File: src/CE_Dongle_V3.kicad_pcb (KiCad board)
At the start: 4 copper layers, 44 x 44 mm, 110 parts, among them J1 USB_C_Receptacle_USB2.0_16P, J2 8P8C_LED_Shielded, J3 Conn_Coaxial, J4 Conn_02x05_Odd_Even, J5 Conn_01x02, Q1 AO3401A, Q2 AO3401A, Q3 BC817-40-7-F, Q4 BC817-40-7-F, Q5 BC817-40-7-F, U1 ESP32-C6, U10 TMUX1208QRSVRQ1, U11 TPS70950DBVR, U2 SP3485, U3 W25Q64JWUUIQ, U4 TPS54302DDCR, U5 PCF8574RGTR(UMW), U6 PCF8574RGTR(UMW), U7 TMUX1208QRSVRQ1, U8 TMUX1208QRSVRQ1, U9 TMUX1208QRSVRQ1, Y1 40MHz

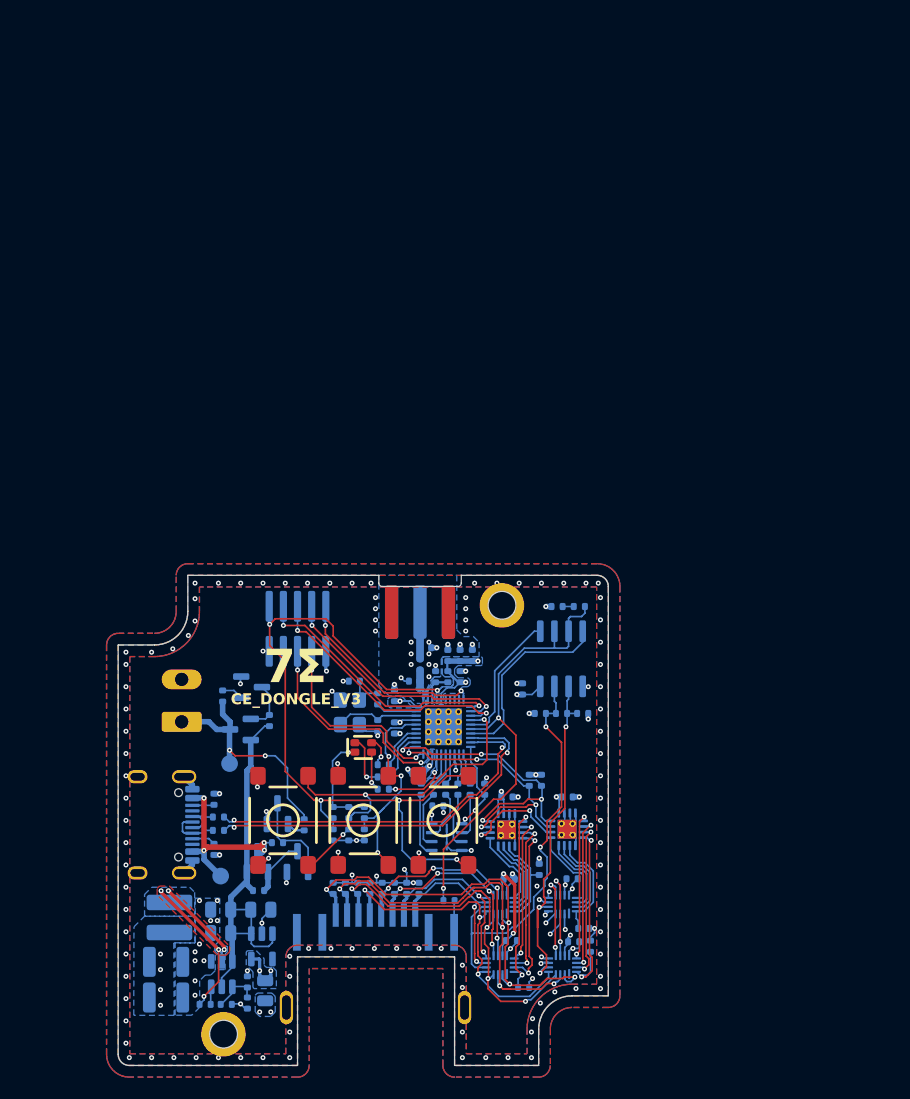
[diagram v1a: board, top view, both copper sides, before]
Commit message: ongoing work
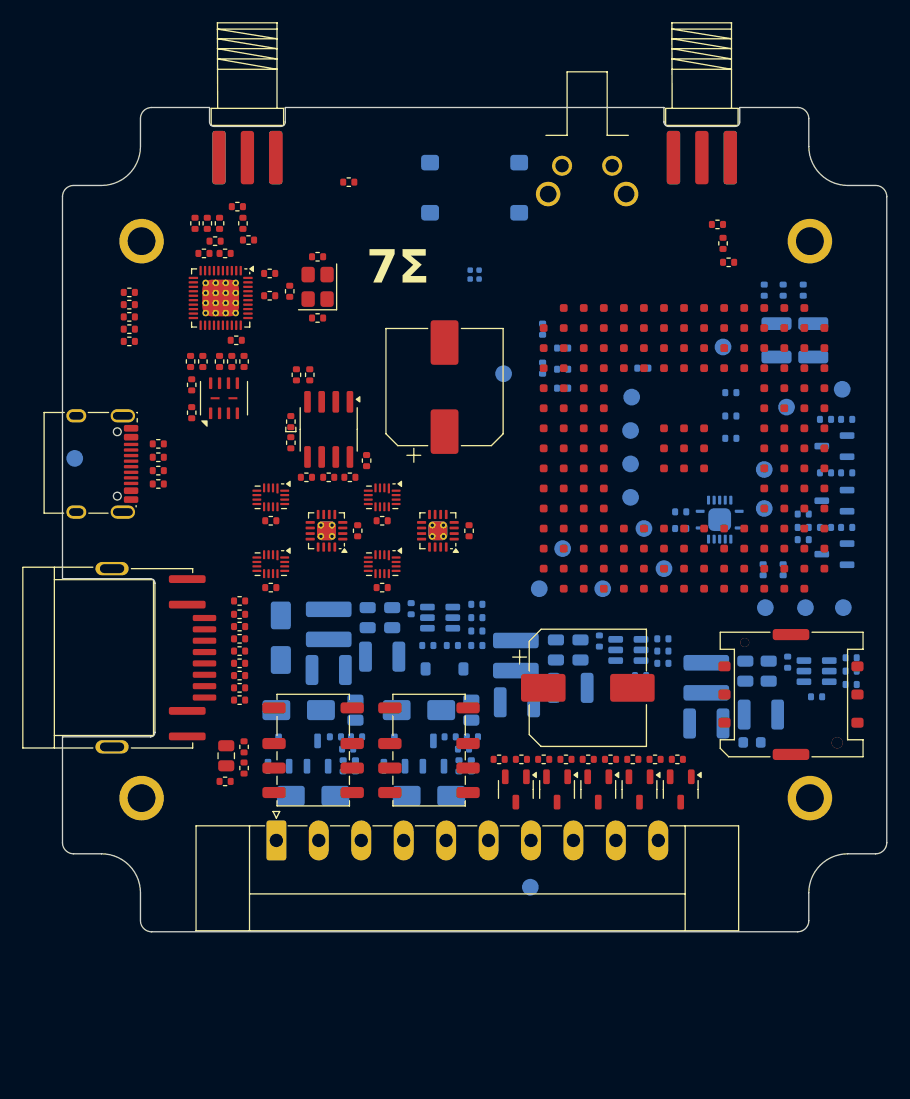
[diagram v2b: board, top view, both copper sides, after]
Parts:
- removed D7: XL-3227SURUGC, 7Sigma:LED-SMD_4P-L1.6-W1.5-BR
- removed G2: Hammond_1551RFLGY, 7Sigma:HAMMOND_1551RFLGY
- removed J2: 8P8C_LED_Shielded, 7Sigma:RJ45-TH_RC01812
- removed J3: Conn_Coaxial, 7Sigma:SMA-SMD_BWSMA-KE-P001
- removed Q3, Q4, Q5: BC817-40-7-F, 7Sigma:SOT-23
- removed R19, R23, R24: 120R, 7Sigma:R_0402_1005Metric
- removed R41: 100K, 7Sigma:R_0402_1005Metric
- removed SW_BOOT1, SW_RST1, SW_USR1: KH-6X6X4.3H-STM, 7Sigma:SW-SMD_4P-L6.0-W6.0-P4.50-LS9.0-H4.3
- removed U11: TPS70950DBVR, 7Sigma:SOT-23-5
- added C40: 100nF, 7Sigma:C_0402_1005Metric, B.Cu at (170.7, 115.9)
- added C41: 220pF, 7Sigma:C_0402_1005Metric, B.Cu at (173.8, 113.6)
- added C42: 47uF, 7Sigma:C_1210_3225Metric, B.Cu at (160.8, 118.3)
- added C43: 47uF, 7Sigma:C_1210_3225Metric, B.Cu at (165.7, 117.5)
- added C44: 470uF, 7Sigma:CP_Elec_10x10, F.Cu at (150.2, 115.1)
- added C45: 470uF, 7Sigma:CP_Elec_10x10, F.Cu at (137.3, 88.1)
- added C48: 100nF, 7Sigma:C_0402_1005Metric, B.Cu at (166.0, 79.4)
- added C49: 100nF, 7Sigma:C_0402_1005Metric, B.Cu at (167.7, 79.4)
- added C50: 100nF, 7Sigma:C_0402_1005Metric, B.Cu at (158.5, 99.3)
- added C51: 100nF, 7Sigma:C_0402_1005Metric, B.Cu at (158.5, 100.8)
- added C52: 10nF, 7Sigma:C_0402_1005Metric, B.Cu at (169.5, 101.8)
- added C53: 10nF, 7Sigma:C_0402_1005Metric, B.Cu at (169.5, 99.5)
- added C54: 100nF, 7Sigma:C_0402_1005Metric, B.Cu at (169.5, 79.4)
- added C62: 33pF, 7Sigma:C_0402_1005Metric, B.Cu at (167.7, 104.5)
- added C63: 33pF, 7Sigma:C_0402_1005Metric, B.Cu at (165.9, 104.5)
- added C64: 1uF, 7Sigma:C_0402_1005Metric, B.Cu at (146.1, 82.9)
- added C65: 33pF, 7Sigma:C_0402_1005Metric, B.Cu at (147.9, 88.2)
- added C66: 100nF, 7Sigma:C_0402_1005Metric, B.Cu at (147.9, 84.6)
- added C67: 33pF, 7Sigma:C_0402_1005Metric, B.Cu at (163.0, 88.6)
- added C68: 33pF, 7Sigma:C_0402_1005Metric, B.Cu at (163.0, 90.7)
- added C69: 33pF, 7Sigma:C_0402_1005Metric, B.Cu at (163.0, 92.7)
- added C70: 1.2pF, 7Sigma:C_0402_1005Metric, F.Cu at (162.8, 76.9)
- added C71: 1.2pF, 7Sigma:C_0402_1005Metric, F.Cu at (161.8, 73.5)
- added C78: 47uF, 7Sigma:C_1210_3225Metric, B.Cu at (167.1, 83.9)
- added C79: 47uF, 7Sigma:C_1210_3225Metric, B.Cu at (170.4, 83.9)
- added C80: 10uF, 7Sigma:C_0805_2012Metric, B.Cu at (129.3, 117.1)
- added C81: 100nF, 7Sigma:C_0402_1005Metric, B.Cu at (135.8, 111.3)
- added C82: 100pF, 7Sigma:C_0402_1005Metric, B.Cu at (140.2, 107.6)
- added C83: 47uF, 7Sigma:C_1210_3225Metric, B.Cu at (131.7, 112.3)
- added C84: 10uF, 7Sigma:C_0805_2012Metric, B.Cu at (139.7, 117.1)
- added C85: 10uF, 7Sigma:C_0805_2012Metric, B.Cu at (147.3, 111.7)
- added C86: 10uF, 7Sigma:C_0805_2012Metric, B.Cu at (149.5, 111.7)
- added C87: 10uF, 7Sigma:C_0805_2012Metric, B.Cu at (130.4, 108.8)
- added C90: 100nF, 7Sigma:C_0402_1005Metric, B.Cu at (151.2, 110.9)
- added C91: 100nF, 7Sigma:C_0402_1005Metric, B.Cu at (168.1, 112.8)
- added C92: 100nF, 7Sigma:C_0402_1005Metric, B.Cu at (134.3, 108.0)
- added C93: 47uF, 7Sigma:C_1210_3225Metric, B.Cu at (126.9, 113.5)
- added D1: SMAJ28CA, 7Sigma:D_SMA, B.Cu at (125.5, 124.8)
- added D10: SMAJ28CA, 7Sigma:D_SMA, B.Cu at (135.9, 124.8)
- added D11: SS34, 7Sigma:D_SMA, B.Cu at (122.6, 110.6)
- added D12: 5V1, 7Sigma:D_SOD-123, B.Cu at (137.3, 113.4)
- added D3: LTST-C281KRKT, 7Sigma:LED_0402_1005Metric, B.Cu at (169.5, 100.7)
- added D5: LTST-C281KRKT, 7Sigma:LED_0402_1005Metric, B.Cu at (129.4, 119.5)
- added D6: SS34, 7Sigma:D_SMA, B.Cu at (124.2, 117.1)
- added D8: LTST-C281KRKT, 7Sigma:LED_0402_1005Metric, B.Cu at (139.8, 119.5)
- added D9: SS34, 7Sigma:D_SMA, B.Cu at (135.0, 117.1)
- added ENC1: Hammond_1551XFLGY, 7Sigma:HAMMOND_1551XFLGY, F.Cu at (140.0, 100.0)
- added FB1: 68nH, 7Sigma:L_0603_1608Metric, B.Cu at (164.9, 120.0)
- added H3: MH_2.5mm_4mm_OD, 7Sigma:MountingHole_2.5mm_Pad_4mm, F.Cu at (170.1, 125.0)
- added H4: MH_2.5mm_4mm_OD, 7Sigma:MountingHole_2.5mm_Pad_4mm, F.Cu at (170.1, 75.0)
- added J7: 8P8C_LED_Shielded, 7Sigma:RJ45-TH_RC01812, F.Cu at (111.6, 112.4)
- added J8: DB2ERM-3.81-10P-GN, 7Sigma:PhoenixContact_MC_1,5_10-GF-3.81_1x10_P3.81mm_Horizontal_ThreadedFlange, F.Cu at (122.2, 128.8)
- added J9: SIM_NANO_Socket, 7Sigma:SIM-SMD_NANO-SIM-TL6P-H1.35, F.Cu at (168.4, 115.7)
- added K1: G6K-2F-Y-TR DC5, 7Sigma:RELAY-SMD_G6K-2F-X-XX, F.Cu at (125.5, 120.7)
- added K2: G6K-2F-Y-TR DC5, 7Sigma:RELAY-SMD_G6K-2F-X-XX, F.Cu at (135.9, 120.7)
- added L5: 4.7uH, 7Sigma:L_Changjiang_FTC404030S, B.Cu at (160.8, 114.2)
- added L6: 4.7uH, 7Sigma:L_Changjiang_FTC404030S, B.Cu at (126.9, 109.4)
- added LP1: FIX-LEMB2-4.8V0-F, 7Sigma:FIX-LEMB2-4.8V0-F, B.Cu at (140.0, 78.0)
- added Q11: SI2308A, 7Sigma:SOT-23-3, F.Cu at (151.1, 124.2)
- added Q12: SI2308A, 7Sigma:SOT-23-3, F.Cu at (154.8, 124.2)
- added Q13: SI2308A, 7Sigma:SOT-23-3, F.Cu at (147.4, 124.2)
- added Q14: SI2308A, 7Sigma:SOT-23-3, B.Cu at (136.3, 121.0)
- added Q15: SI2308A, 7Sigma:SOT-23-3, B.Cu at (125.9, 121.0)
- added Q16: SI2308A, 7Sigma:SOT-23-3, B.Cu at (132.8, 121.0)
- added Q17: SI2308A, 7Sigma:SOT-23-3, B.Cu at (122.4, 121.0)
- added Q18: SI2308A, 7Sigma:SOT-23-3, B.Cu at (172.3, 103.1)
- added Q7: BC817-40-7-F, 7Sigma:SOT-23-3, B.Cu at (172.3, 98.3)
- added Q8: BC817-40-7-F, 7Sigma:SOT-23-3, B.Cu at (172.3, 93.4)
- added R20: 120R, 7Sigma:R_0402_1005Metric, B.Cu at (171.5, 100.7)
- added R31: 10K, 7Sigma:R_0402_1005Metric, F.Cu at (109.0, 81.8)
- added R33: 100K, 7Sigma:R_0402_1005Metric, B.Cu at (173.4, 95.8)
- added R34: 100K, 7Sigma:R_0402_1005Metric, B.Cu at (173.4, 91.0)
- added R35: 10K, 7Sigma:R_0402_1005Metric, B.Cu at (171.5, 95.8)
- added R36: 10K, 7Sigma:R_0402_1005Metric, B.Cu at (171.5, 91.0)
- added R45: 10K, 7Sigma:R_0402_1005Metric, B.Cu at (147.9, 86.5)
- added R46: 0R, 7Sigma:R_0402_1005Metric, F.Cu at (162.3, 75.2)
- added R47: 100K, 7Sigma:R_0402_1005Metric, B.Cu at (173.4, 100.7)
- added R48: 22K, 7Sigma:R_0402_1005Metric, F.Cu at (144.2, 121.5)
- added R49: 5K1, 7Sigma:R_0402_1005Metric, F.Cu at (119.3, 122.3)
- added R50: 120R, 7Sigma:R_0805_2012Metric, F.Cu at (117.7, 121.2)
- added R51: 10K, 7Sigma:R_0402_1005Metric, B.Cu at (146.1, 86.4)
- added R52: 10K, 7Sigma:R_0402_1005Metric, B.Cu at (155.1, 86.4)
- added R55: 22K, 7Sigma:R_0402_1005Metric, F.Cu at (148.2, 121.5)
- added R56: 22K, 7Sigma:R_0402_1005Metric, F.Cu at (158.2, 121.5)
- added R57: 10K, 7Sigma:R_0402_1005Metric, B.Cu at (128.6, 120.6)
- added R58: 162K, 7Sigma:R_0402_1005Metric, B.Cu at (140.2, 110.0)
- added R59: 22K, 7Sigma:R_0402_1005Metric, B.Cu at (140.2, 108.8)
- added R6: 22K, 7Sigma:R_0402_1005Metric, B.Cu at (173.8, 112.4)
- added R60: 10K, 7Sigma:R_0402_1005Metric, B.Cu at (139.0, 120.6)
- added R61: 10K, 7Sigma:R_0402_1005Metric, B.Cu at (138.6, 122.1)
- added R62: 100K, 7Sigma:R_0402_1005Metric, B.Cu at (139.7, 122.1)
- added R69: 10K, 7Sigma:R_0402_1005Metric, B.Cu at (129.3, 122.1)
- added R7: 118K, 7Sigma:R_0402_1005Metric, B.Cu at (173.8, 114.8)
- added R70: 100K, 7Sigma:R_0402_1005Metric, B.Cu at (128.2, 122.1)
- added R71: 22K, 7Sigma:R_0402_1005Metric, F.Cu at (156.2, 121.5)
- added R72: 22K, 7Sigma:R_0402_1005Metric, F.Cu at (150.2, 121.5)
- added SW1: TC-6615-9.0-160G, 7Sigma:SW-TH_4P-RA-L6.0-W6.0-H9.0, F.Cu at (150.1, 69.5)
- added SW2: KH-6X6X7H-STM, 7Sigma:SW-SMD_4P-L6.0-W6.0-P4.50-LS9.0-H7.0, B.Cu at (140.0, 70.2)
- added TP10: TestPoint, 7Sigma:TestPoint_Pad_D1.5mm, B.Cu at (157.0, 104.4)
- added TP11: TestPoint, 7Sigma:TestPoint_Pad_D1.5mm, B.Cu at (166.1, 107.9)
- added TP12: TestPoint, 7Sigma:TestPoint_Pad_D1.5mm, B.Cu at (162.3, 84.5)
- added TP13: TestPoint, 7Sigma:TestPoint_Pad_D1.5mm, B.Cu at (154.0, 98.0)
- added TP14: TestPoint, 7Sigma:TestPoint_Pad_D1.5mm, B.Cu at (173.0, 88.3)
- added TP15: TestPoint, 7Sigma:TestPoint_Pad_D1.5mm, B.Cu at (169.7, 107.9)
- added TP16: TestPoint, 7Sigma:TestPoint_Pad_D1.5mm, B.Cu at (173.1, 107.9)
- added TP17: TestPoint, 7Sigma:TestPoint_Pad_D1.5mm, B.Cu at (155.2, 100.8)
- added TP18: TestPoint, 7Sigma:TestPoint_Pad_D1.5mm, B.Cu at (166.0, 95.5)
- added TP19: TestPoint, 7Sigma:TestPoint_Pad_D1.5mm, B.Cu at (166.0, 99.0)
- added TP20: TestPoint, 7Sigma:TestPoint_Pad_D1.5mm, B.Cu at (142.6, 86.9)
- added TP21: TestPoint, 7Sigma:TestPoint_Pad_D1.5mm, B.Cu at (154.0, 95.0)
- added TP22: TestPoint, 7Sigma:TestPoint_Pad_D1.5mm, B.Cu at (154.0, 92.0)
- added TP23: TestPoint, 7Sigma:TestPoint_Pad_D1.5mm, B.Cu at (154.1, 89.0)
- added TP24: TestPoint, 7Sigma:TestPoint_Pad_D1.5mm, B.Cu at (168.0, 89.9)
- added TP7: TestPoint, 7Sigma:TestPoint_Pad_D1.5mm, B.Cu at (147.9, 102.6)
- added TP8: TestPoint, 7Sigma:TestPoint_Pad_D1.5mm, B.Cu at (145.8, 106.2)
- added TP9: TestPoint, 7Sigma:TestPoint_Pad_D1.5mm, B.Cu at (151.5, 106.2)
- added U14: TPS54302DDCR, 7Sigma:SOT-23-6, B.Cu at (170.7, 113.6)
- added U15: TXS0104ERGYR, 7Sigma:VQFN-14_L3.5-W3.5-P0.50-BL-EP, B.Cu at (162.0, 100.0)
- added U16: LE910R1, 7Sigma:XCVR_LE910R1-EU, F.Cu at (158.8, 93.6)
- added U17: WS2812, 7Sigma:LED-SMD_4P-L1.3-W1.3-P0.80_WS2812E-1313, B.Cu at (140.0, 78.0)
- added U19: TPS54302DDCR, 7Sigma:SOT-23-6, B.Cu at (136.9, 108.8)
- C1, C10, C11, C12, C13, C14, C15, C16, C17, C18, C25, C26, C27, C28, C29, C30, C31, C32, C33, C34, C35, C36, C37, C38, C39, C4, C6, C7, C8, C9, D2, J1, L1, L2, R1, R10, R11, R12, R13, R14, R15, R16, R17, R18, R21, R22, R26, R27, R28, R3, R4, R42, R43, R8, R9, U1, U10, U2, U3, U5, U6, U7, U8, U9, Y1: moved to F.Cu
- C22: value 10uF -> 1uF; footprint 7Sigma:C_0805_2012Metric -> 7Sigma:C_0402_1005Metric; moved to F.Cu
- C24: value 100nF -> 1uF; moved to F.Cu
- J4: value Conn_02x05_Odd_Even -> Conn_Coaxial; footprint 7Sigma:IDC-SMD_10P-P1.27-3220-10-0300-00 -> 7Sigma:SMA-SMD_BWSMA-KE-P001; moved to F.Cu
- J5: value Conn_01x02 -> Conn_Coaxial; footprint 7Sigma:PhoenixContact_MC_1,5_2-G-3.81_1x02_P3.81mm_Horizontal -> 7Sigma:SMA-SMD_BWSMA-KE-P001; moved to F.Cu
- Q1, Q2: footprint 7Sigma:SOT-23 -> 7Sigma:SOT-23-3; moved to F.Cu
- R29: value 100K -> 1K; moved to F.Cu
- R30: value 120R -> 5K1; moved to F.Cu
- R37, R38, R40: value 10K -> 374K
- R39: value 10K -> 100K
- R44: value 10K -> 120R; moved to F.Cu
- R5: value 120R -> 1K; moved to F.Cu
- moved C22 73.0 mm to (128.7, 69.7), turned to 0 degrees
- moved H1 71.6 mm to (110.1, 75.0)
- moved J4 55.7 mm to (160.4, 67.5), turned to 90 degrees
- moved C2 54.5 mm to (166.4, 113.6), turned to -90 degrees
- moved C25 52.0 mm to (109.0, 79.6), turned to 180 degrees
- moved C23 51.7 mm to (164.3, 113.6), turned to -90 degrees
- moved J5 51.0 mm to (119.6, 67.5)
- moved C8 50.5 mm to (115.7, 76.1)
- moved C20 49.7 mm to (156.9, 112.9)
- moved C26 49.5 mm to (109.0, 82.9), turned to 180 degrees
- moved R21 49.1 mm to (109.0, 80.7), turned to 0 degrees
- moved C19 49.0 mm to (154.9, 114.0)
- moved R25 48.9 mm to (156.9, 111.8), turned to 180 degrees
- moved R2 48.4 mm to (156.9, 110.7), turned to 0 degrees
- moved U10 46.8 mm to (121.7, 98.0), turned to -90 degrees
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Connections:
- net Net-(U1-XTAL_N) renamed /MCU/XTAL_N
- net Net-(U1-XTAL_P) renamed /MCU/XTAL_P
- net VDD_SPI renamed /MCU/VDD_SPI
- C15 pad 1: Net-(J3-In) -> Net-(J5-In)
- C22 pad 1: 5V0 -> 3V3
- C24 pad 1: /MCU/BTTN -> /MISC/TEMP_VCC
- C26 pad 1: /MCU/GPIO8_BOOT -> /MCU/BUTTON
- J4 pad 1: 3V3 -> /LTE/RF_ANT
- J4 pad 2: /MCU/MTMS -> GND
- J5 pad 1: /PWR/VEXT -> Net-(J5-In)
- L2 pad 1: Net-(J3-In) -> Net-(J5-In)
- Q2 pad 1: Net-(Q2-G) -> /PWR/nSOURCE_USB
- R22 pad 2: /MCU/GPIO8_BOOT -> /MCU/BUTTON
- R27 pad 1: /PWR/VSUPPLY -> Net-(Q1-G)
- R27 pad 2: Net-(Q1-G) -> Net-(Q13-D)
- R28 pad 1: /PWR/VBUS -> Net-(Q11-D)
- R28 pad 2: Net-(Q4-C) -> GND
- R29 pad 1: /PWR/VSUPPLY -> Net-(J7-Pad11)
- R29 pad 2: Net-(Q2-G) -> GND
- R30 pad 1: Net-(J2-Pad12) -> GND
- R30 pad 2: /TX_EN -> Net-(Q11-G)
- R37 pad 1: /MUX/MUX_0_EN -> /PWR/VSUPPLY
- R37 pad 2: GND -> Net-(D12-K)
- R38 pad 1: /MUX/MUX_1_EN -> /MISC/RY2_CTRL
- R39 pad 1: /MUX/MUX_2_EN -> Net-(D12-K)
- R40 pad 1: /MUX/MUX_3_EN -> /MISC/RY1_CTRL
- R44 pad 1: 3V3 -> /MISC/TEMP_DATA
- R44 pad 2: /MCU/BTTN -> /MISC/TEMP
- U1 pad 10: /MCU/MTMS -> /LTE/PWR_CYCLE
- U1 pad 11: /MCU/MTDI -> /LTE/UART_TX
- U1 pad 12: /MCU/MTCK -> /LTE/UART_RX
- U1 pad 13: /MCU/MTDO -> /LTE/PWR_MON
- U1 pad 14: /MCU/GPIO8_BOOT -> /MCU/GPIO8
- U1 pad 15: /MCU/MB_RX -> /MCU/BUTTON
- U1 pad 27: /MCU/LED_B -> /MCU/MB_RX
- U1 pad 33: /MCU/LED_R -> /MISC/RY1_CTRL
- U1 pad 34: /MCU/LED_G -> /MISC/RY2_CTRL
- U1 pad 36: /MCU/BTTN -> unconnected-(U1-SDIO_DATA3-Pad36)
- U1 pad 7: unconnected-(U1-XTAL_32K_N-Pad7) -> /LTE/SHUTDOWN
- U1 pad 8: unconnected-(U1-GPIO2-Pad8) -> /MISC/TEMP
- U1 pad 9: unconnected-(U1-GPIO3-Pad9) -> /MCU/LED_DATA
- U4 pad 5: /PWR/VSUPPLY -> unconnected-(U4-EN-Pad5)
- U5 pad 14: /MUX/I2C_nINT -> unconnected-(U5-~{INT}-Pad14)
- U6 pad 14: /MUX/I2C_nINT -> unconnected-(U6-~{INT}-Pad14)
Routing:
- net 3V3: track 139.6 -> 0.00 mm, vias 17 -> 0
- net /MCU/RST: track 65.8 -> 0.00 mm, vias 5 -> 0
- net GND: track 62.5 -> 0.00 mm, vias 163 -> 0
- net 5V0: track 55.2 -> 0.00 mm, vias 6 -> 0
- net /MUX/IN_1: track 47.6 -> 0.00 mm, vias 5 -> 0
- net /MUX/IN_2: track 45.1 -> 0.00 mm, vias 5 -> 0
- net /MUX/IN_3: track 42.5 -> 0.00 mm, vias 5 -> 0
- net /TX_EN: track 40.7 -> 0.00 mm, vias 2 -> 0
- net /MUX/IN_4: track 37.7 -> 0.00 mm, vias 4 -> 0
- net /MUX/OUT_B: track 37.0 -> 0.00 mm, vias 2 -> 0
- net /PWR/VSUPPLY: track 36.3 -> 0.00 mm
- net /MUX/IN_5: track 35.7 -> 0.00 mm, vias 6 -> 0
- net /MCU/USB_D-: track 33.9 -> 0.00 mm, vias 2 -> 0
- net /MCU/GPIO8_BOOT: track 33.2 -> 0.00 mm, vias 3 -> 0
- net /MCU/USB_D+: track 32.8 -> 0.00 mm, vias 2 -> 0
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- removed copper zone on B.Cu, net 3V3
- removed copper zone on B.Cu, net 5V0
- removed copper zone on B.Cu, net GND
- removed copper zone on F.Cu, net GND
- removed copper zone on In1.Cu, net GND
- removed copper zone on In2.Cu, net GND
- removed copper zone on B.Cu, net Net-(C10-Pad1)
- removed copper zone on B.Cu, net Net-(U1-ANT)
- removed copper zone on B.Cu, net Net-(U4-SW)
- removed copper zone on F.Cu, net Net-(U4-SW)
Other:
- board size 44 x 44 mm -> 74 x 74 mm
- board text removed: "CE_DONGLE_V3"
